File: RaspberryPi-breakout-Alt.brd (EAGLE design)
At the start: 33.5 x 41.7 mm, 3 parts

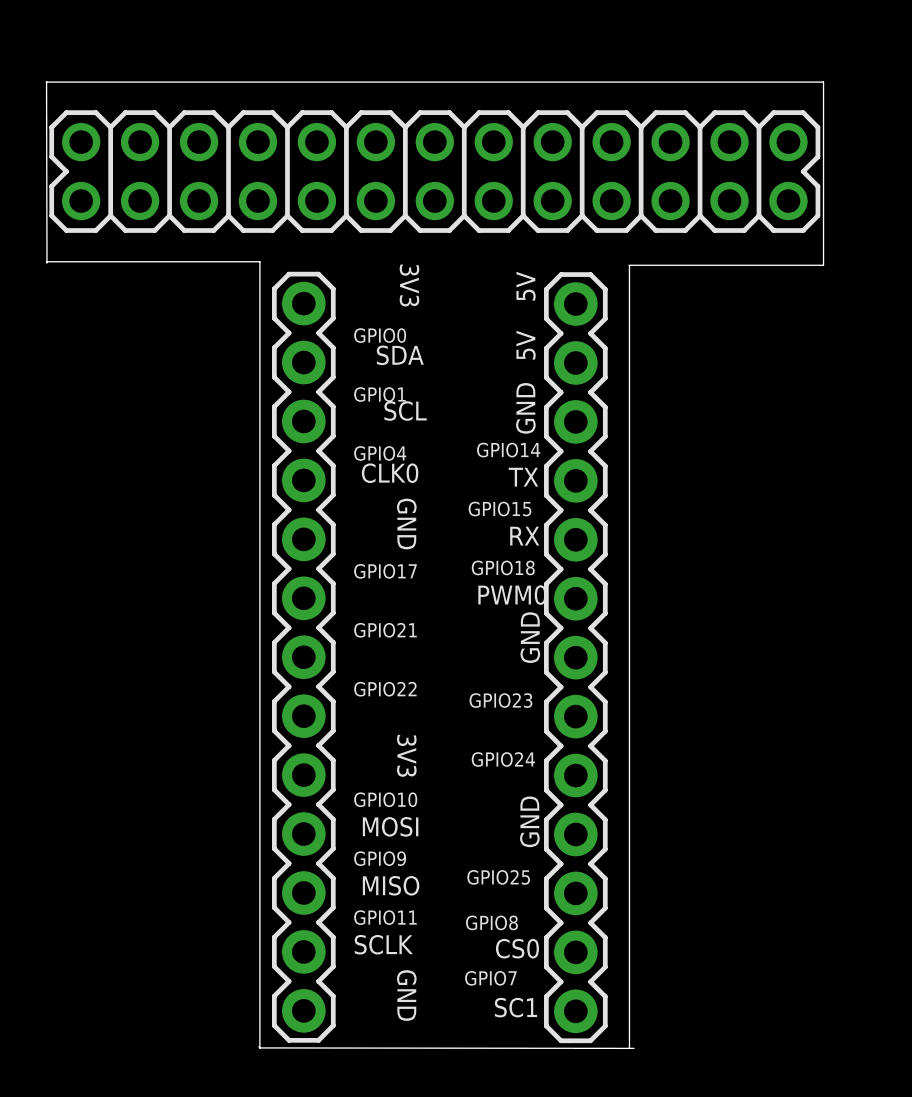
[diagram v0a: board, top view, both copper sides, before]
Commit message: Created a new board
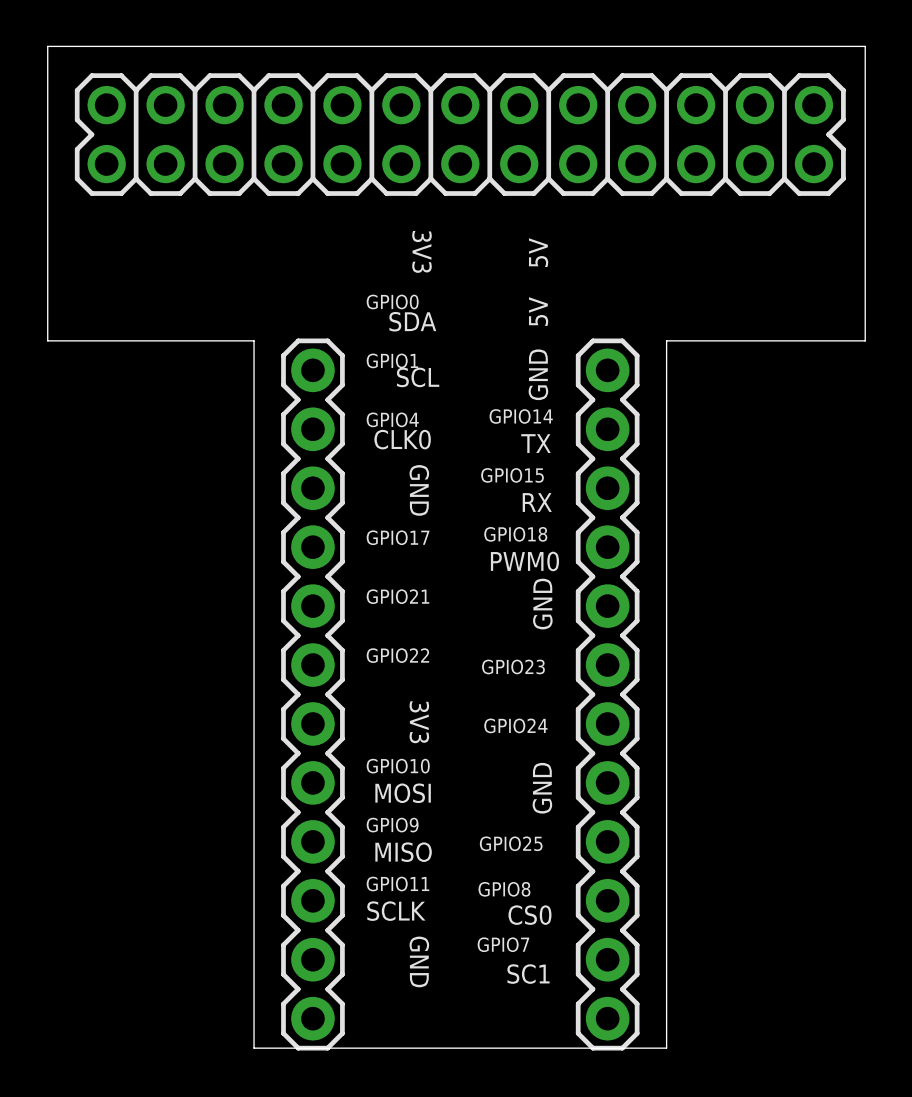
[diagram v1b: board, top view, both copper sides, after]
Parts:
- removed JP2, JP3: (no value), SparkFun-Connectors:1X13
- added JP4, JP5: (no value), SparkFun-Connectors:1X12
- moved JP1 1.94 mm to (2.54, 38.1)
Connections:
- removed net N$1: JP1.2, JP3.1
- removed net N$13: JP1.26, JP3.13
- removed net N$14: JP1.25, JP2.13
- removed net N$15: JP1.23, JP2.12
- removed net N$2: JP1.4, JP3.2
- removed net N$25: JP1.3, JP2.2
- removed net N$26: JP1.1, JP2.1
- removed net N$3: JP1.6, JP3.3
- new net 3V3_A: JP1.1, JP4.11
- new net 3V3_B: JP1.17, JP5.11
- new net 5V_A: JP1.2, JP4.10
- new net 5V_B: JP1.4, JP5.10
- new net CLK0-G4: JP1.7
- new net CS0-G8: JP1.24
- new net G17: JP1.11
- new net G21: JP1.13
- new net G22: JP1.15
- new net G23: JP1.16
- new net G24: JP1.18
- new net G25: JP1.22
- new net GND_A: JP1.9, JP4.12
- new net GND_B: JP1.25, JP5.12
- new net GND_C: JP1.6
- new net GND_D: JP1.14
- new net GND_E: JP1.20
- new net MISO-G9: JP1.21
- new net MOSI-G10: JP1.19
- new net PWM0-G18: JP1.12
- new net RX-G15: JP1.10
- new net SC1-G7: JP1.26
- new net SCKL-G11: JP1.23
- new net SCL-G1: JP1.5
- new net SDA-G0: JP1.3
- new net TX-G14: JP1.8
- net N$10: now also JP4.3; no longer JP1.20, JP3.10
- net N$11: now also JP4.2; no longer JP1.22, JP3.11
- net N$12: now also JP4.1; no longer JP1.24, JP3.12
- net N$16: now also JP5.9; no longer JP1.21, JP2.11
- net N$17: now also JP5.8; no longer JP1.19, JP2.10
- net N$18: now also JP5.7; no longer JP1.17, JP2.9
- net N$19: now also JP5.6; no longer JP1.15, JP2.8
- net N$20: now also JP5.5; no longer JP1.13, JP2.7
- net N$21: now also JP5.4; no longer JP1.11, JP2.6
- net N$22: now also JP5.3; no longer JP1.9, JP2.5
- net N$23: now also JP5.2; no longer JP1.7, JP2.4
- net N$24: now also JP5.1; no longer JP1.5, JP2.3
- net N$4: now also JP4.9; no longer JP1.8, JP3.4
- net N$5: now also JP4.8; no longer JP1.10, JP3.5
- net N$6: now also JP4.7; no longer JP1.12, JP3.6
- net N$7: now also JP4.6; no longer JP1.14, JP3.7
- net N$8: now also JP4.5; no longer JP1.16, JP3.8
- net N$9: now also JP4.4; no longer JP1.18, JP3.9
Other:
- board size 33.5 x 41.7 mm -> 35.2 x 43.2 mm
